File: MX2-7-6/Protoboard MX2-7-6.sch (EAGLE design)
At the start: 139 parts, among them CN1 1X4-CLEANBIG, CN2 1X4-CLEANBIG, CN3 1X4-CLEANBIG, J1 DCJ0202

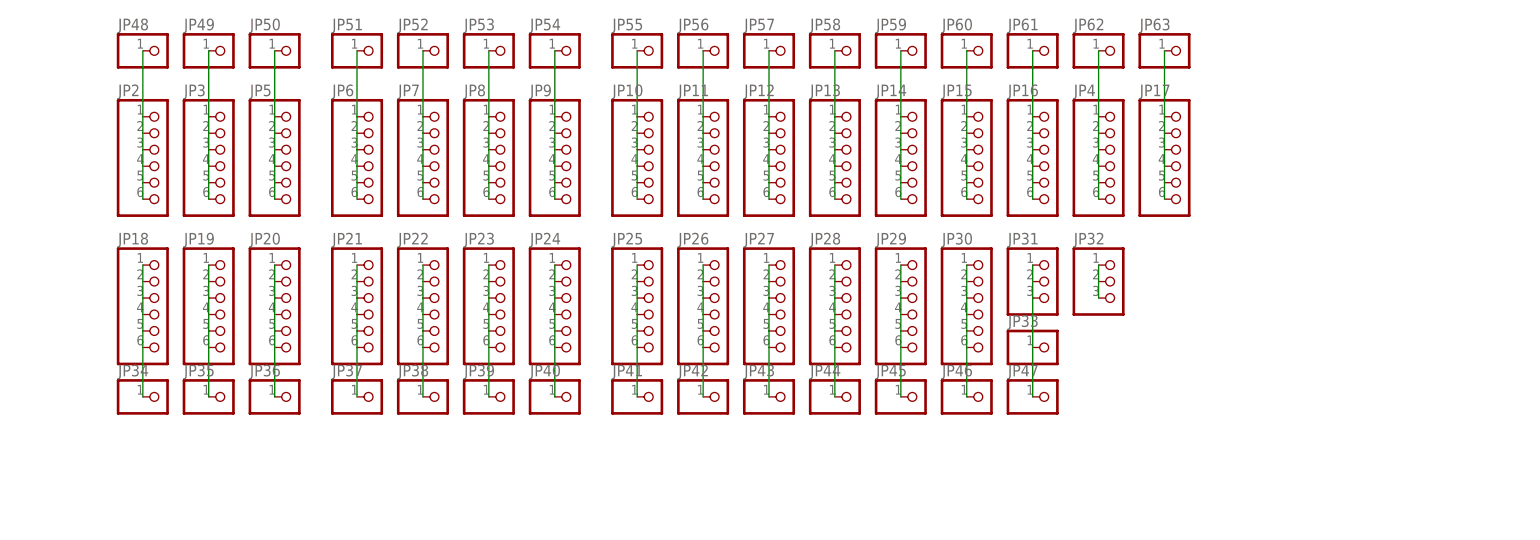
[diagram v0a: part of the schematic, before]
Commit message: Update esp component and usb
test
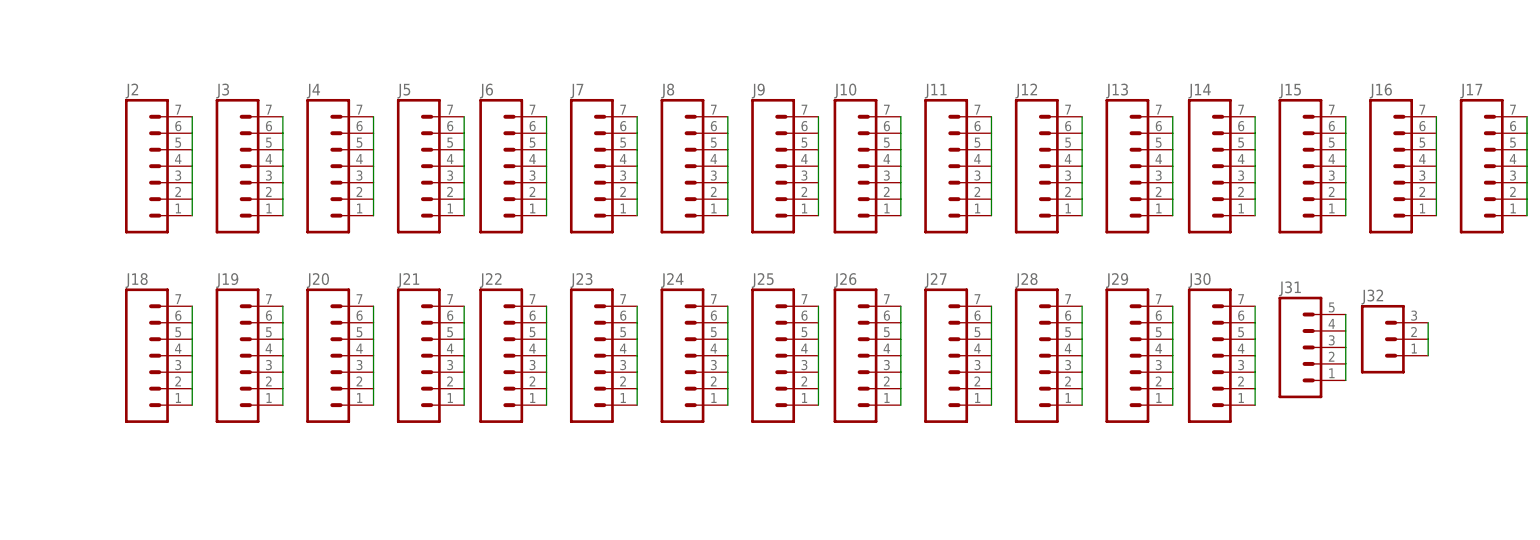
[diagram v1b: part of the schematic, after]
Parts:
- removed JP10, JP11, JP12, JP13, JP14, JP15, JP16, JP17, JP18, JP19, JP2, JP20, JP21, JP22, JP23, JP24, JP25, JP26, JP27, JP28, JP29, JP3, JP30, JP4, JP5, JP6, JP7, JP8, JP9: (no value), adafruit:PINHD-1X6CB
- removed JP31, JP32: (no value), adafruit:PINHD-1X3CB
- removed JP33, JP34, JP35, JP36, JP37, JP38, JP39, JP40, JP41, JP42, JP43, JP44, JP45, JP46, JP47, JP48, JP49, JP50, JP51, JP52, JP53, JP54, JP55, JP56, JP57, JP58, JP59, JP60, JP61, JP62, JP63: (no value), adafruit:PINHD-1X1CB
- added J10, J11, J12, J13, J14, J15, J16, J17, J18, J19, J2, J20, J21, J22, J23, J24, J25, J26, J27, J28, J29, J3, J30, J4, J5, J6, J7, J8, J9: (no value), SparkFun-Connectors:M07NO_SILK
- added J31: (no value), SparkFun-Connectors:M05NO_SILK
- added J32: (no value), SparkFun-Connectors:M031X03_NO_SILK
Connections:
- net N$1: now also J2.1, J2.2, J2.3, J2.4, J2.5, J2.6, J2.7; no longer JP2.1, JP2.2, JP2.3, JP2.4, JP2.5, JP2.6, JP48.1
- net N$10: now also J8.1, J8.2, J8.3, J8.4, J8.5, J8.6, J8.7; no longer JP54.1, JP9.1, JP9.2, JP9.3, JP9.4, JP9.5, JP9.6
- net N$11: now also J9.1, J9.2, J9.3, J9.4, J9.5, J9.6, J9.7; no longer JP10.1, JP10.2, JP10.3, JP10.4, JP10.5, JP10.6, JP55.1
- net N$12: now also J10.1, J10.2, J10.3, J10.4, J10.5, J10.6, J10.7; no longer JP11.1, JP11.2, JP11.3, JP11.4, JP11.5, JP11.6, JP56.1
- net N$13: now also J11.1, J11.2, J11.3, J11.4, J11.5, J11.6, J11.7; no longer JP12.1, JP12.2, JP12.3, JP12.4, JP12.5, JP12.6, JP57.1
- net N$14: now also J12.1, J12.2, J12.3, J12.4, J12.5, J12.6, J12.7; no longer JP13.1, JP13.2, JP13.3, JP13.4, JP13.5, JP13.6, JP58.1
- net N$15: now also J13.1, J13.2, J13.3, J13.4, J13.5, J13.6, J13.7; no longer JP14.1, JP14.2, JP14.3, JP14.4, JP14.5, JP14.6, JP59.1
- net N$16: now also J14.1, J14.2, J14.3, J14.4, J14.5, J14.6, J14.7; no longer JP15.1, JP15.2, JP15.3, JP15.4, JP15.5, JP15.6, JP60.1
- net N$17: now also J15.1, J15.2, J15.3, J15.4, J15.5, J15.6, J15.7; no longer JP16.1, JP16.2, JP16.3, JP16.4, JP16.5, JP16.6, JP61.1
- net N$18: now also J16.1, J16.2, J16.3, J16.4, J16.5, J16.6, J16.7; no longer JP4.1, JP4.2, JP4.3, JP4.4, JP4.5, JP4.6, JP62.1
- net N$19: now also J17.1, J17.2, J17.3, J17.4, J17.5, J17.6, J17.7; no longer JP17.1, JP17.2, JP17.3, JP17.4, JP17.5, JP17.6, JP63.1
- net N$20: now also J18.1, J18.2, J18.3, J18.4, J18.5, J18.6, J18.7; no longer JP18.1, JP18.2, JP18.3, JP18.4, JP18.5, JP18.6, JP34.1
- net N$21: now also J19.1, J19.2, J19.3, J19.4, J19.5, J19.6, J19.7; no longer JP19.1, JP19.2, JP19.3, JP19.4, JP19.5, JP19.6, JP35.1
- net N$22: now also J20.1, J20.2, J20.3, J20.4, J20.5, J20.6, J20.7; no longer JP20.1, JP20.2, JP20.3, JP20.4, JP20.5, JP20.6, JP36.1
- net N$27: now also J21.1, J21.2, J21.3, J21.4, J21.5, J21.6, J21.7; no longer JP21.1, JP21.2, JP21.3, JP21.4, JP21.5, JP21.6, JP37.1
- net N$28: now also J22.1, J22.2, J22.3, J22.4, J22.5, J22.6, J22.7; no longer JP22.1, JP22.2, JP22.3, JP22.4, JP22.5, JP22.6, JP38.1
- net N$29: now also J23.1, J23.2, J23.3, J23.4, J23.5, J23.6, J23.7; no longer JP23.1, JP23.2, JP23.3, JP23.4, JP23.5, JP23.6, JP39.1
- net N$30: now also J24.1, J24.2, J24.3, J24.4, J24.5, J24.6, J24.7; no longer JP24.1, JP24.2, JP24.3, JP24.4, JP24.5, JP24.6, JP40.1
- net N$31: now also J25.1, J25.2, J25.3, J25.4, J25.5, J25.6, J25.7; no longer JP25.1, JP25.2, JP25.3, JP25.4, JP25.5, JP25.6, JP41.1
- net N$32: now also J26.1, J26.2, J26.3, J26.4, J26.5, J26.6, J26.7; no longer JP26.1, JP26.2, JP26.3, JP26.4, JP26.5, JP26.6, JP42.1
- net N$33: now also J27.1, J27.2, J27.3, J27.4, J27.5, J27.6, J27.7; no longer JP27.1, JP27.2, JP27.3, JP27.4, JP27.5, JP27.6, JP43.1
- net N$35: now also J28.1, J28.2, J28.3, J28.4, J28.5, J28.6, J28.7; no longer JP28.1, JP28.2, JP28.3, JP28.4, JP28.5, JP28.6, JP44.1
- net N$36: now also J29.1, J29.2, J29.3, J29.4, J29.5, J29.6, J29.7; no longer JP29.1, JP29.2, JP29.3, JP29.4, JP29.5, JP29.6, JP45.1
- net N$37: now also J30.1, J30.2, J30.3, J30.4, J30.5, J30.6, J30.7; no longer JP30.1, JP30.2, JP30.3, JP30.4, JP30.5, JP30.6, JP46.1
- net N$38: now also J31.1, J31.2, J31.3, J31.4, J31.5; no longer JP31.1, JP31.2, JP31.3, JP33.1, JP47.1
- net N$39: now also J32.1, J32.2, J32.3; no longer JP32.1, JP32.2, JP32.3
- net N$5: now also J3.1, J3.2, J3.3, J3.4, J3.5, J3.6, J3.7; no longer JP3.1, JP3.2, JP3.3, JP3.4, JP3.5, JP3.6, JP49.1
- net N$6: now also J4.1, J4.2, J4.3, J4.4, J4.5, J4.6, J4.7; no longer JP5.1, JP5.2, JP5.3, JP5.4, JP5.5, JP5.6, JP50.1
- net N$7: now also J5.1, J5.2, J5.3, J5.4, J5.5, J5.6, J5.7; no longer JP51.1, JP6.1, JP6.2, JP6.3, JP6.4, JP6.5, JP6.6
- net N$8: now also J6.1, J6.2, J6.3, J6.4, J6.5, J6.6, J6.7; no longer JP52.1, JP7.1, JP7.2, JP7.3, JP7.4, JP7.5, JP7.6
- net N$9: now also J7.1, J7.2, J7.3, J7.4, J7.5, J7.6, J7.7; no longer JP53.1, JP8.1, JP8.2, JP8.3, JP8.4, JP8.5, JP8.6
